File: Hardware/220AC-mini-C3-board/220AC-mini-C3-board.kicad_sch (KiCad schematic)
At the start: 23 parts, among them J1 AC MAINS POWER, J2 ON/OFF switch, J3 Conn_01x04, K1 HF163-F, Q1 Q_NPN_CBE, Q2 Q_NPN_CBE, U1 PBO-3C-3

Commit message: 220AC 3.3DC adapter redesigned 1.1
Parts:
- K1: footprint footprint:HF163FL24HL2T -> footprint:FH44L-1AT-L2-DC3V; LCSC C140724 -> C498276
- L1: footprint footprint:SMDRI127-470MT -> footprint:IND_BRL3225T4R7M; LCSC C24548 -> C454090
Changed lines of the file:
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@@
     (property "Reference" "L1" (id 0) (at 175.26 59.2922 90))
     (property "Value" "L" (id 1) (at 175.26 61.8291 90))
-    (property "Footprint" "footprint:SMDRI127-470MT" (id 2) (at 175.26 63.5 0)
-      (effects (font (size 1.27 1.27)) hide)
-    )
-    (property "Datasheet" "https://jlcpcb.com/partdetail/25288-SMDRI1274R7NT/C24548" (id 3) (at 175.26 63.5 0)
-      (effects (font (size 1.27 1.27)) hide)
-    )
-    (property "LCSC" "C24548" (id 4) (at 175.26 63.5 90)
+    (property "Footprint" "footprint:IND_BRL3225T4R7M" (id 2) (at 175.26 63.5 0)
+      (effects (font (size 1.27 1.27)) hide)
+    )
+    (property "Datasheet" "https://www.lcsc.com/product-detail/Inductors-SMD_Taiyo-Yuden-BRL3225T4R7M_C454090.html" (id 3) (at 175.26 63.5 0)
+      (effects (font (size 1.27 1.27)) hide)
+    )
+    (property "LCSC" "C454090" (id 4) (at 175.26 63.5 90)
       (effects (font (size 1.27 1.27)) hide)
     )
@@
   )
   (symbol (lib_id "Device:C_Polarized") (at 91.44 77.47 0) (unit 1)
-    (in_bom yes) (on_board yes) (fields_autoplaced)
+    (in_bom yes) (on_board no) (fields_autoplaced)
     (property "Reference" "C1" (id 0) (at 94.361 76.6353 0)
       (effects (font (size 1.27 1.27)) (justify left))
@@
       (effects (font (size 1.27 1.27)) (justify left))
     )
-    (property "Footprint" "footprint:HF163FL24HL2T" (id 2) (at 148.59 123.19 0)
-      (effects (font (size 1.27 1.27)) hide)
-    )
-    (property "Datasheet" "https://jlcpcb.com/partdetail/152050-HF163F_L_3HL2T/C140724" (id 3) (at 148.59 123.19 0)
-      (effects (font (size 1.27 1.27)) hide)
-    )
-    (property "LCSC" "C140724" (id 4) (at 148.59 123.19 0)
+    (property "Footprint" "footprint:FH44L-1AT-L2-DC3V" (id 2) (at 148.59 123.19 0)
+      (effects (font (size 1.27 1.27)) hide)
+    )
+    (property "Datasheet" "https://www.lcsc.com/product-detail/_Zhejiang-Fanhar-_C498276.html" (id 3) (at 148.59 123.19 0)
+      (effects (font (size 1.27 1.27)) hide)
+    )
+    (property "LCSC" "C498276" (id 4) (at 148.59 123.19 0)
       (effects (font (size 1.27 1.27)) hide)
     )
@@
   )
   (symbol (lib_id "Mechanical:MountingHole") (at 77.47 124.46 0) (unit 1)
-    (in_bom yes) (on_board yes) (fields_autoplaced)
+    (in_bom yes) (on_board no) (fields_autoplaced)
     (property "Reference" "H2" (id 0) (at 80.01 123.5515 0)
       (effects (font (size 1.27 1.27)) (justify left))
@@
   )
   (symbol (lib_id "Mechanical:MountingHole") (at 77.47 132.08 0) (unit 1)
-    (in_bom yes) (on_board yes) (fields_autoplaced)
+    (in_bom yes) (on_board no) (fields_autoplaced)
     (property "Reference" "H4" (id 0) (at 80.01 131.2453 0)
       (effects (font (size 1.27 1.27)) (justify left))
@@
     )
     (path "/98ed8559-0b85-40d0-9540-9691164c3fca"
-      (reference "K1") (unit 1) (value "HF163-F") (footprint "footprint:HF163FL24HL2T")
+      (reference "K1") (unit 1) (value "HF163-F") (footprint "footprint:FH44L-1AT-L2-DC3V")
     )
     (path "/491f8f1b-4139-4a25-93c5-d945ce211f8c"
-      (reference "L1") (unit 1) (value "L") (footprint "footprint:SMDRI127-470MT")
+      (reference "L1") (unit 1) (value "L") (footprint "footprint:IND_BRL3225T4R7M")
     )
     (path "/876d6114-7ceb-4ab2-9410-592e876bfa77"

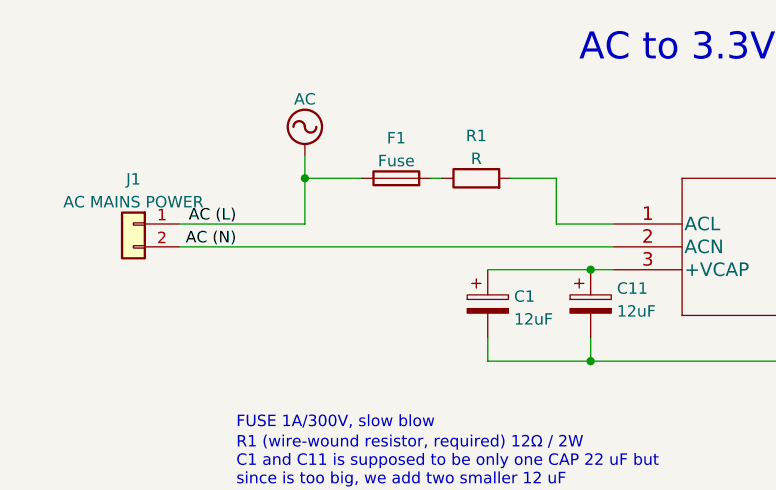
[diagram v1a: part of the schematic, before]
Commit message: cambios CAF
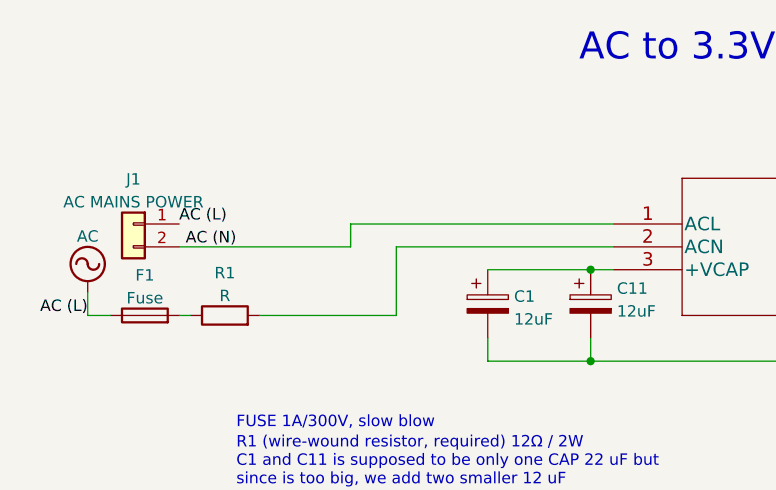
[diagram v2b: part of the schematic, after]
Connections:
- net AC (N): now also U1.1 (ACL); no longer U1.2 (ACN)
- net at R1.2: now also U1.2 (ACN); no longer U1.1 (ACL)
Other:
- moved on the sheet: F1, R1
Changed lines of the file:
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@@
   (junction (at 102.87 73.66) (diameter 0) (color 0 0 0 0)
   )
-  (junction (at 71.12 63.5) (diameter 0) (color 0 0 0 0)
-  )
   (junction (at 184.15 63.5) (diameter 0) (color 0 0 0 0)
   )
@@
     (stroke (width 0) (type default) (color 0 0 0 0))
   )
-  (wire (pts (xy 99.06 68.58) (xy 105.41 68.58))
-    (stroke (width 0) (type default) (color 0 0 0 0))
-  )
   (wire (pts (xy 151.13 130.81) (xy 151.13 140.97))
     (stroke (width 0) (type default) (color 0 0 0 0))
   )
-  (wire (pts (xy 57.15 71.12) (xy 105.41 71.12))
-    (stroke (width 0) (type default) (color 0 0 0 0))
-  )
   (wire (pts (xy 158.75 110.49) (xy 158.75 115.57))
     (stroke (width 0) (type default) (color 0 0 0 0))
@@
     (stroke (width 0) (type default) (color 0 0 0 0))
   )
-  (wire (pts (xy 99.06 63.5) (xy 99.06 68.58))
+  (wire (pts (xy 81.28 71.12) (xy 105.41 71.12))
     (stroke (width 0) (type default) (color 0 0 0 0))
   )
@@
     (stroke (width 0) (type default) (color 0 0 0 0))
   )
-  (wire (pts (xy 71.12 60.96) (xy 71.12 63.5))
+  (wire (pts (xy 46.99 76.2) (xy 46.99 78.74))
     (stroke (width 0) (type default) (color 0 0 0 0))
   )
@@
     (stroke (width 0) (type default) (color 0 0 0 0))
   )
+  (wire (pts (xy 76.2 71.12) (xy 76.2 68.58))
+    (stroke (width 0) (type default) (color 0 0 0 0))
+  )
   (wire (pts (xy 156.21 68.58) (xy 160.02 68.58))
     (stroke (width 0) (type default) (color 0 0 0 0))
@@
     (stroke (width 0) (type default) (color 0 0 0 0))
   )
-  (wire (pts (xy 93.98 63.5) (xy 99.06 63.5))
+  (wire (pts (xy 66.04 78.74) (xy 81.28 78.74))
     (stroke (width 0) (type default) (color 0 0 0 0))
   )
@@
     (stroke (width 0) (type default) (color 0 0 0 0))
   )
+  (wire (pts (xy 57.15 71.12) (xy 76.2 71.12))
+    (stroke (width 0) (type default) (color 0 0 0 0))
+  )
   (wire (pts (xy 165.1 73.66) (xy 165.1 71.12))
     (stroke (width 0) (type default) (color 0 0 0 0))
@@
     (stroke (width 0) (type default) (color 0 0 0 0))
   )
-  (wire (pts (xy 71.12 63.5) (xy 77.47 63.5))
+  (wire (pts (xy 81.28 78.74) (xy 81.28 71.12))
     (stroke (width 0) (type default) (color 0 0 0 0))
   )
@@
     (stroke (width 0) (type default) (color 0 0 0 0))
   )
+  (wire (pts (xy 46.99 78.74) (xy 49.53 78.74))
+    (stroke (width 0) (type default) (color 0 0 0 0))
+  )
   (wire (pts (xy 222.25 73.66) (xy 229.87 73.66))
     (stroke (width 0) (type default) (color 0 0 0 0))
   )
-  (wire (pts (xy 85.09 63.5) (xy 86.36 63.5))
-    (stroke (width 0) (type default) (color 0 0 0 0))
-  )
-  (wire (pts (xy 57.15 68.58) (xy 71.12 68.58))
+  (wire (pts (xy 57.15 78.74) (xy 58.42 78.74))
     (stroke (width 0) (type default) (color 0 0 0 0))
   )
@@
     (stroke (width 0) (type default) (color 0 0 0 0))
   )
-  (wire (pts (xy 71.12 63.5) (xy 71.12 68.58))
-    (stroke (width 0) (type default) (color 0 0 0 0))
-  )
   (wire (pts (xy 217.17 73.66) (xy 222.25 73.66))
     (stroke (width 0) (type default) (color 0 0 0 0))
@@
   )
   (polyline (pts (xy 232.41 76.2) (xy 232.41 87.63))
+    (stroke (width 0) (type default) (color 0 0 0 0))
+  )
+  (wire (pts (xy 76.2 68.58) (xy 105.41 68.58))
     (stroke (width 0) (type default) (color 0 0 0 0))
   )
@@
     (effects (font (size 1.27 1.27)) (justify right bottom))
   )
-  (label "AC (L)" (at 63.5 68.58 180)
-    (effects (font (size 1.27 1.27)) (justify right bottom))
+  (label "AC (L)" (at 57.15 68.58 0)
+    (effects (font (size 1.27 1.27)) (justify left bottom))
   )
   (label "IO_2" (at 203.2 132.08 0)
@@
   )
   (label "IO_2" (at 208.28 78.74 180)
+    (effects (font (size 1.27 1.27)) (justify right bottom))
+  )
+  (label "AC (L)" (at 46.99 78.74 180)
     (effects (font (size 1.27 1.27)) (justify right bottom))
   )
@@
     (pin "2")
   )
-  (symbol (lib_id "Device:R") (at 90.17 63.5 90) (unit 1)
-    (in_bom yes) (on_board yes) (fields_autoplaced)
-    (property "Reference" "R1" (id 0) (at 90.17 58.7842 90))
-    (property "Value" "R" (id 1) (at 90.17 61.3211 90))
-    (property "Footprint" "footprint:SMW212RJT" (id 2) (at 90.17 65.278 90)
-      (effects (font (size 1.27 1.27)) hide)
-    )
-    (property "Datasheet" "https://jlcpcb.com/partdetail/TeConnectivity-SMW212RJT/C2073396" (id 3) (at 90.17 63.5 0)
-      (effects (font (size 1.27 1.27)) hide)
-    )
-    (property "LCSC" "C2073396" (id 4) (at 90.17 63.5 90)
+  (symbol (lib_id "Device:R") (at 62.23 78.74 90) (unit 1)
+    (in_bom yes) (on_board yes) (fields_autoplaced)
+    (property "Reference" "R1" (id 0) (at 62.23 74.0242 90))
+    (property "Value" "R" (id 1) (at 62.23 76.5611 90))
+    (property "Footprint" "footprint:SMW212RJT" (id 2) (at 62.23 80.518 90)
+      (effects (font (size 1.27 1.27)) hide)
+    )
+    (property "Datasheet" "https://jlcpcb.com/partdetail/TeConnectivity-SMW212RJT/C2073396" (id 3) (at 62.23 78.74 0)
+      (effects (font (size 1.27 1.27)) hide)
+    )
+    (property "LCSC" "C2073396" (id 4) (at 62.23 78.74 90)
       (effects (font (size 1.27 1.27)) hide)
     )
@@
     (pin "3")
   )
-  (symbol (lib_id "power:AC") (at 71.12 60.96 0) (unit 1)
-    (in_bom yes) (on_board yes) (fields_autoplaced)
-    (property "Reference" "#PWR01" (id 0) (at 71.12 63.5 0)
-      (effects (font (size 1.27 1.27)) hide)
-    )
-    (property "Value" "AC" (id 1) (at 71.12 54.7172 0))
-    (property "Footprint" "" (id 2) (at 71.12 60.96 0)
-      (effects (font (size 1.27 1.27)) hide)
-    )
-    (property "Datasheet" "" (id 3) (at 71.12 60.96 0)
+  (symbol (lib_id "power:AC") (at 46.99 76.2 0) (unit 1)
+    (in_bom yes) (on_board yes) (fields_autoplaced)
+    (property "Reference" "#PWR01" (id 0) (at 46.99 78.74 0)
+      (effects (font (size 1.27 1.27)) hide)
+    )
+    (property "Value" "AC" (id 1) (at 46.99 69.9572 0))
+    (property "Footprint" "" (id 2) (at 46.99 76.2 0)
+      (effects (font (size 1.27 1.27)) hide)
+    )
+    (property "Datasheet" "" (id 3) (at 46.99 76.2 0)
       (effects (font (size 1.27 1.27)) hide)
     )
@@
     (pin "5")
   )
-  (symbol (lib_id "Device:Fuse") (at 81.28 63.5 90) (unit 1)
-    (in_bom yes) (on_board yes) (fields_autoplaced)
-    (property "Reference" "F1" (id 0) (at 81.28 59.0382 90))
-    (property "Value" "Fuse" (id 1) (at 81.28 61.5751 90))
-    (property "Footprint" "footprint:0443001.DR" (id 2) (at 81.28 65.278 90)
-      (effects (font (size 1.27 1.27)) hide)
-    )
-    (property "Datasheet" "https://jlcpcb.com/partdetail/Littelfuse-0443001DR/C95352" (id 3) (at 81.28 63.5 0)
-      (effects (font (size 1.27 1.27)) hide)
-    )
-    (property "LCSC" "C95352" (id 4) (at 81.28 63.5 90)
-      (effects (font (size 1.27 1.27)) hide)
-    )
+  (symbol (lib_id "Device:Fuse") (at 53.34 78.74 90) (unit 1)
+    (in_bom yes) (on_board yes) (fields_autoplaced)
+    (property "Reference" "F1" (id 0) (at 53.34 74.2782 90))
+    (property "Value" "Fuse" (id 1) (at 53.34 76.8151 90))
+    (property "Footprint" "footprint:0443001.DR" (id 2) (at 53.34 80.518 90)
+      (effects (font (size 1.27 1.27)) hide)
+    )
+    (property "Datasheet" "https://jlcpcb.com/partdetail/Littelfuse-0443001DR/C95352" (id 3) (at 53.34 78.74 0)
+      (effects (font (size 1.27 1.27)) hide)
+    )
+    (property "LCSC" "C95352" (id 4) (at 53.34 78.74 90)
+      (effects (font (size 1.27 1.27)) hide)
+    )

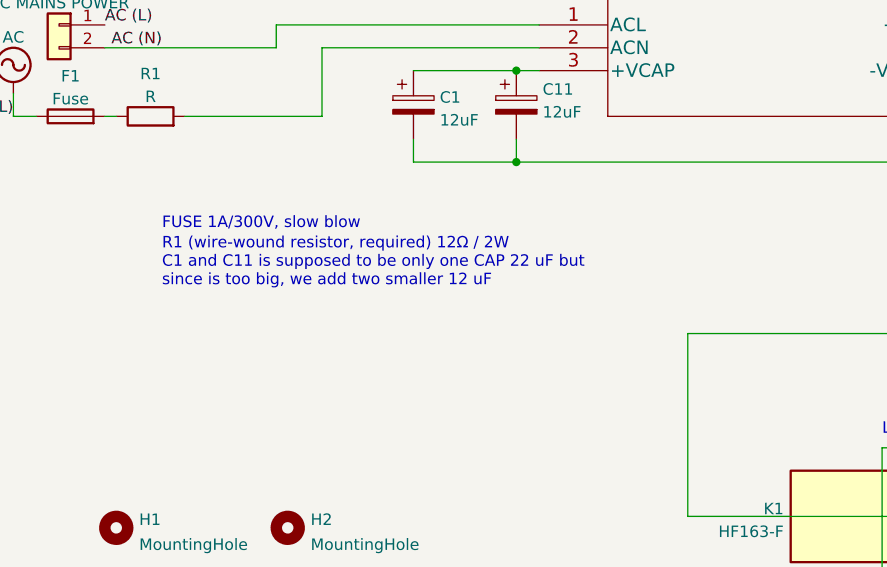
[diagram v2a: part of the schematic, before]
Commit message: Update schematics
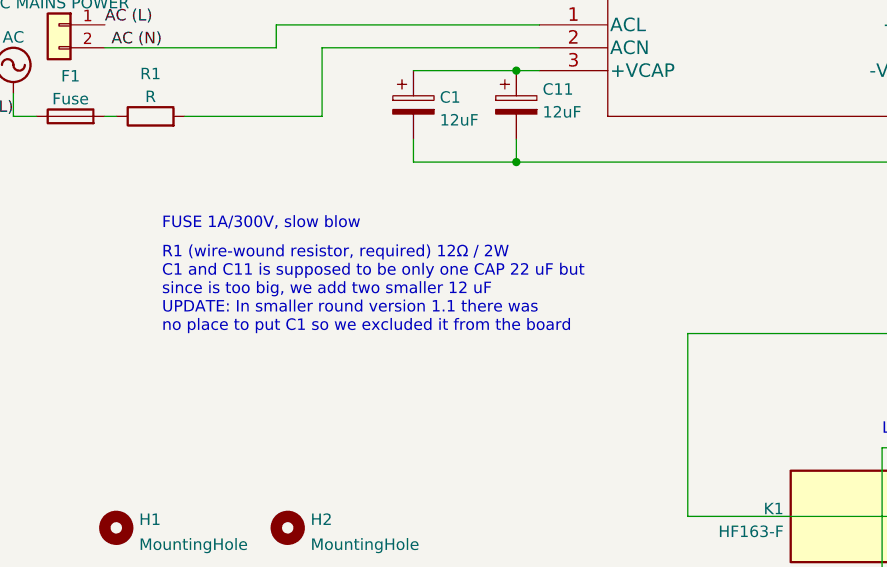
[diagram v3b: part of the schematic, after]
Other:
- note added: "R1 (wire-wound resistor, required) 12Ω / 2W C1 and C11 is supposed to be only one CAP 22 uF but since is too big, we add two smaller 12 uF UPDATE: In smaller round version 1.1 there was no place to put C1 so we excluded it from the board"
- note removed: "R1 (wire-wound resistor, required) 12Ω / 2W C1 and C11 is supposed to be only one CAP 22 uF but since is too big, we add two smaller 12 uF"
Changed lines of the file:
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@@
     (effects (font (size 1.27 1.27)) (justify left bottom))
   )
-  (text "R1 (wire-wound resistor, required) 12Ω / 2W\nC1 and C11 is supposed to be only one CAP 22 uF but\nsince is too big, we add two smaller 12 uF"
-    (at 63.5 97.79 0)
+  (text "R1 (wire-wound resistor, required) 12Ω / 2W\nC1 and C11 is supposed to be only one CAP 22 uF but\nsince is too big, we add two smaller 12 uF\nUPDATE: In smaller round version 1.1 there was\nno place to put C1 so we excluded it from the board"
+    (at 63.5 102.87 0)
     (effects (font (size 1.27 1.27)) (justify left bottom))
   )
